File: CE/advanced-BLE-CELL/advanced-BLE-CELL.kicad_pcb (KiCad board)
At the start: 4 copper layers, 65 x 56 mm, 24 parts, among them J3 40HAT, J6 CONN_02X02, J9 CONN_01X02, Q1 DMG2305UX, Q2 DMMT5401, U1 nRF52840, U2 CAT24C32, U3 BG96

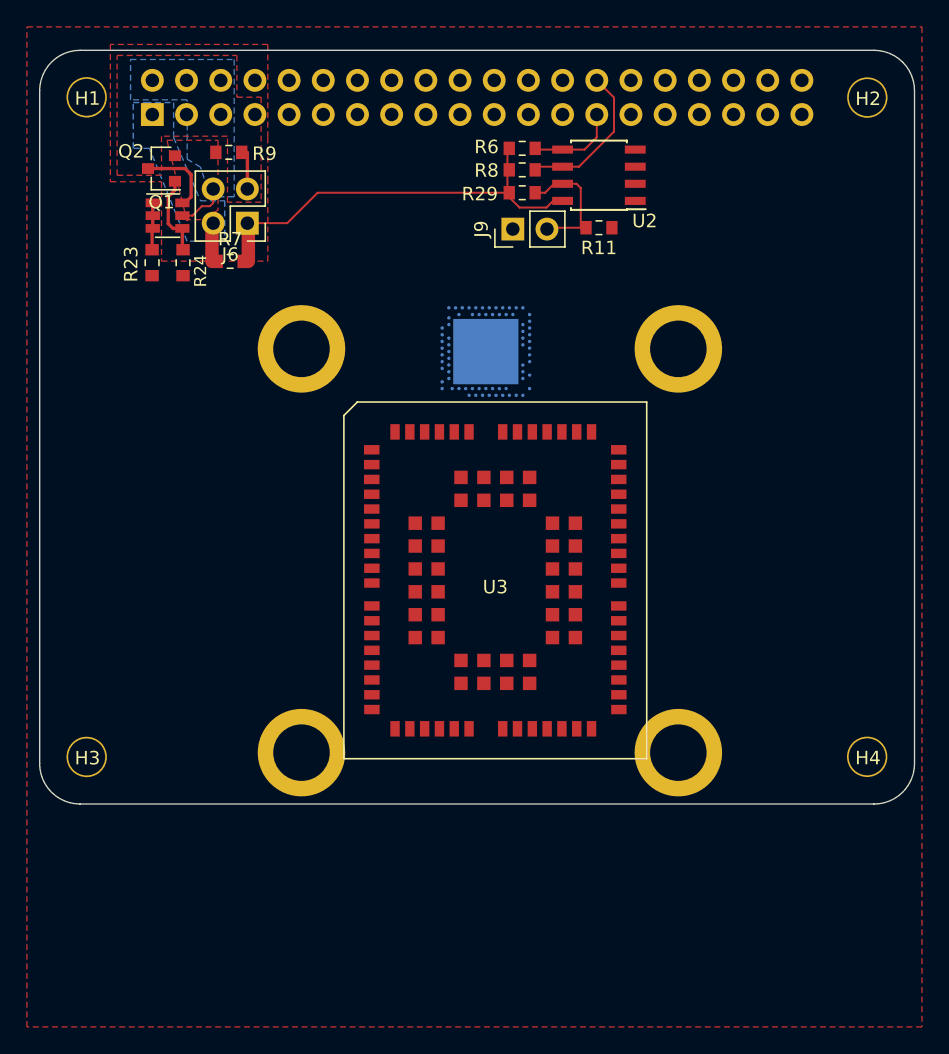
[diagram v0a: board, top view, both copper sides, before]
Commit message: ASFd
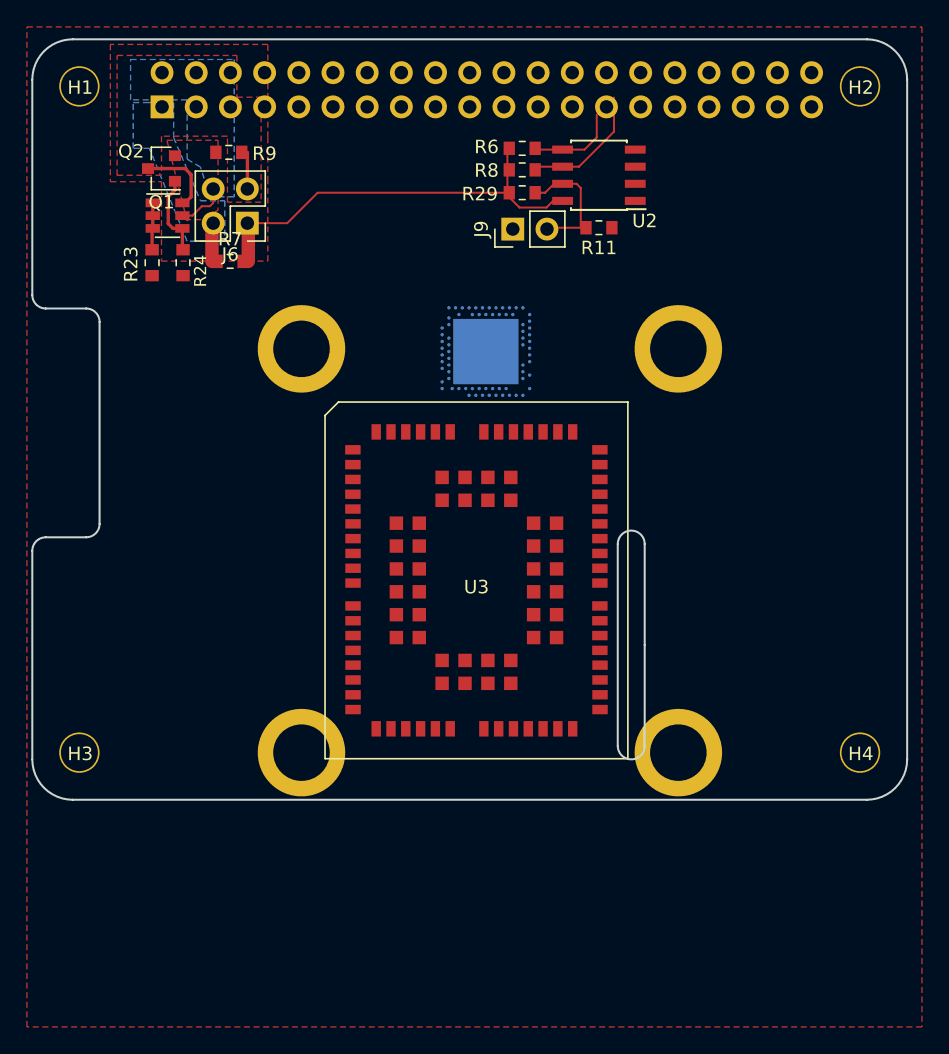
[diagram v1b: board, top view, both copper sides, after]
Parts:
- J3: footprint Connector_PinSocket_2.54mm:PinSocket_2x20_P2.54mm_Vertical -> ABC:PinSocket_2x20_P2.54mm_Vertical-CENTER
- moved J3 23.7 mm to (110.5, 63.8)
- moved U3 1.40 mm to (111.0, 100.2)
- moved H2 0.99 mm to (139.5, 63.5)
- moved H1 0.97 mm to (81.5, 63.5)
- moved H3 0.63 mm to (81.5, 113.0)
- moved H4 0.61 mm to (139.5, 113.0)
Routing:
- net /ID_SC_EEPROM: track 11.7 -> 9.76 mm
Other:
- board size 65 x 56 mm -> 65 x 56.5 mm
